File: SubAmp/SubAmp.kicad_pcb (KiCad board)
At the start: 2 copper layers, 170.4 x 67 mm, 55 parts, among them J1 OUT, J2 VCC, J3 VEE, J4 GND, J6 IN, Q1 MPSA42, Q10 2SA1943, Q11 2SC5200, Q12 2SA1943, Q2 MPSA42, Q3 MPSA42, Q4 MJE15033, Q5 MJE15032, Q6 MJE15033, Q7 2SA1943, Q8 2SC5200, Q9 2SC5200

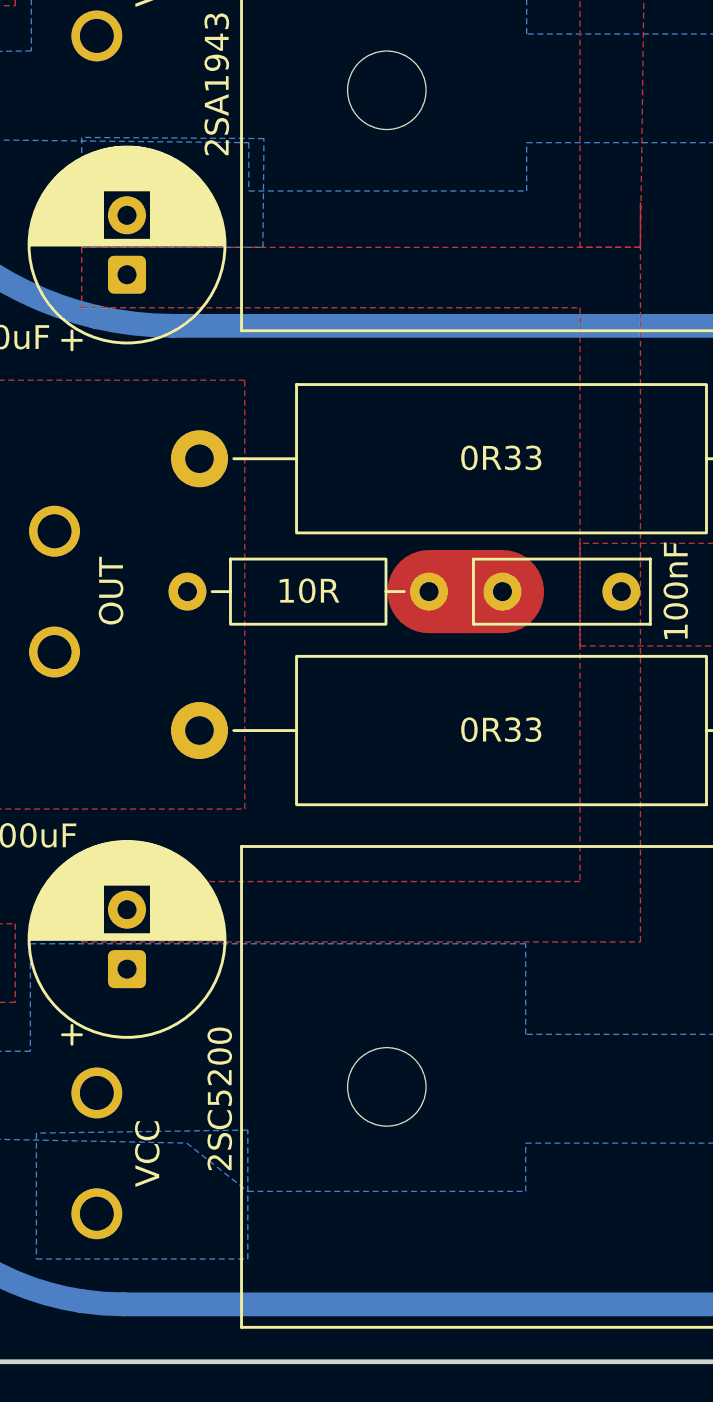
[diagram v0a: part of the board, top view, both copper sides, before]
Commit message: commit
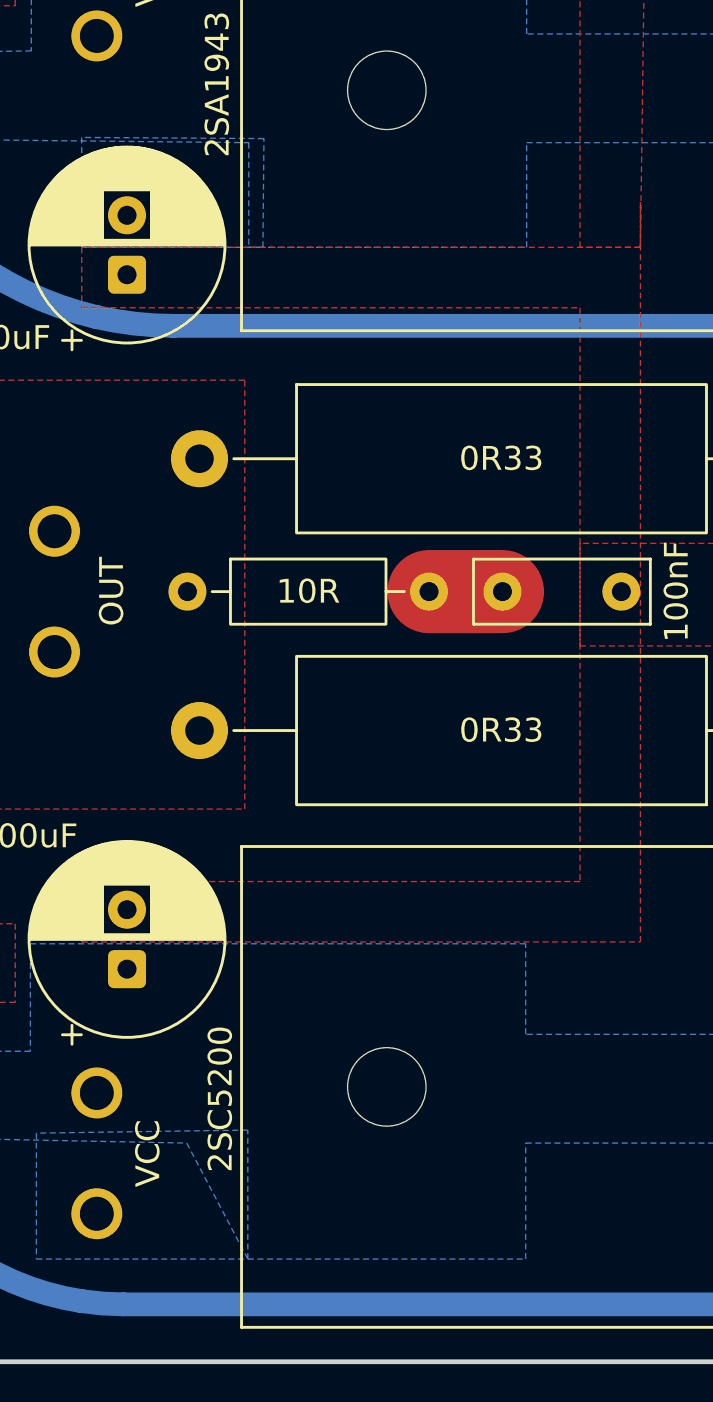
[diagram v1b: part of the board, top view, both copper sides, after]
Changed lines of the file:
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@@
 		(polygon
 			(pts
-				(xy 129.2098 133.7056) (xy 130.3782 132.4356) (xy 131.953 133.8834) (xy 147.291778 134.1882) (xy 149.86 136.2202)
-				(xy 161.544 136.2202) (xy 161.544 134.1882) (xy 183.642 134.1882) (xy 183.642 129.6162) (xy 161.544 129.6162)
+				(xy 129.2098 133.7056) (xy 130.3782 132.4356) (xy 131.953 133.8834) (xy 147.291778 134.1882) (xy 149.86 139.065)
+				(xy 161.544 139.065) (xy 161.544 134.1882) (xy 183.642 134.1882) (xy 183.642 129.6162) (xy 161.544 129.6162)
 				(xy 161.544 125.8062) (xy 140.716 125.8062) (xy 140.716 130.3274) (xy 131.064 130.3274) (xy 130.302 130.6322)
 				(xy 127.4826 131.2164)
@@
 		(polygon
 			(pts
-				(xy 132.1308 90.1446) (xy 130.937 91.186) (xy 131.1148 91.9226) (xy 149.900956 92.118904) (xy 149.900956 94.150904)
-				(xy 161.584956 94.150904) (xy 161.584956 92.118904) (xy 183.682956 92.118904) (xy 183.682956 87.546904)
+				(xy 132.1308 90.1446) (xy 130.937 91.186) (xy 131.1148 91.9226) (xy 149.900956 92.118904) (xy 149.900956 96.52)
+				(xy 161.584956 96.52) (xy 161.584956 92.118904) (xy 183.682956 92.118904) (xy 183.682956 87.546904)
 				(xy 161.584956 87.546904) (xy 161.584956 79.622104) (xy 140.756956 79.622104) (xy 140.756956 88.258104)
 				(xy 131.104956 88.4174) (xy 131.1402 88.4428) (xy 129.9972 88.4936)
